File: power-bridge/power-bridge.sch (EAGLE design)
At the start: 3 parts, among them X2 CON-MA03-2PCB_EDGE

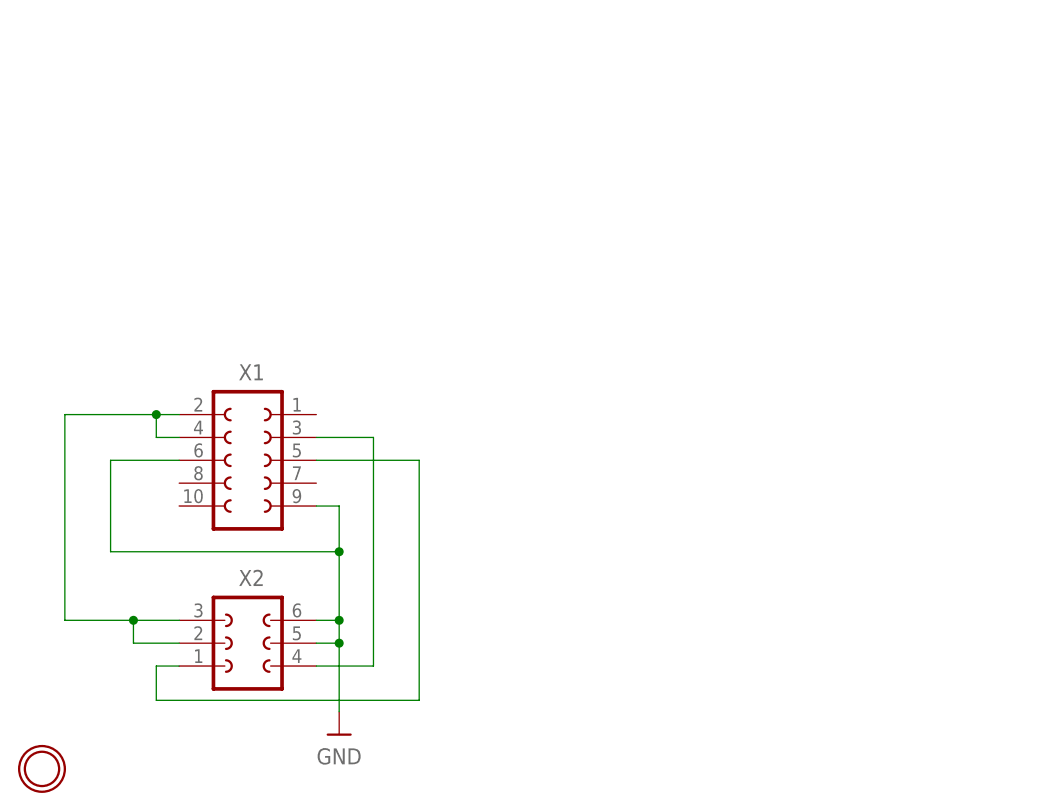
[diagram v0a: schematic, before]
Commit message: Publish v1.0.0 Power Board and Power Bridge
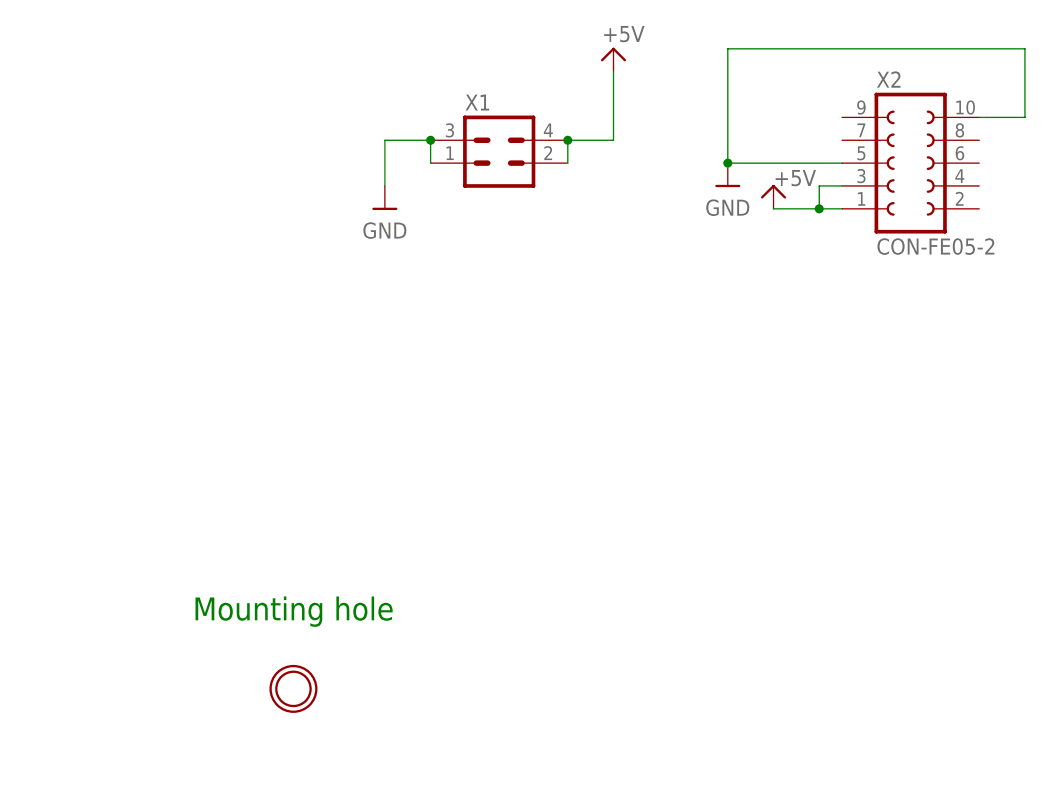
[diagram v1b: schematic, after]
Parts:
- removed U$2: MOUNTINGHOLE2.7_THICK, sanisimov:MOUNTINGHOLE2.7_THICK
- added U$1: MOUNTINGHOLE2.7_THICK, _Library.b1f76137-4d0f-4ce2-9703-0cd83550450f.flbr:MOUNTINGHOLE2.7_THICK
- X1: value (none) -> CON-MA02-2; device sanisimov:CON-FE05-2 -> _Library.b1f76137-4d0f-4ce2-9703-0cd83550450f.flbr:CON-MA02-2
- X2: value CON-MA03-2PCB_EDGE -> CON-FE05-2; device sanisimov:CON-MA03-2PCB_EDGE -> _Library.b1f76137-4d0f-4ce2-9703-0cd83550450f.flbr:CON-FE05-2
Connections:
- removed net N$1: X1.3, X2.4
- removed net N$2: X1.5, X2.1
- removed net PWR: X1.2, X1.4, X2.2, X2.3
- new net +5V: X1.2, X1.4, X2.1, X2.3
- net GND: now also X1.1, X1.3, X2.10; no longer X1.6, X1.9, X2.6
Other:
- note added: "Mounting hole"
